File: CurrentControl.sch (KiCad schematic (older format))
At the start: 8 parts, among them P1 CONN_01X01, P3 A, Q401 BUK9575, U201 LMV358

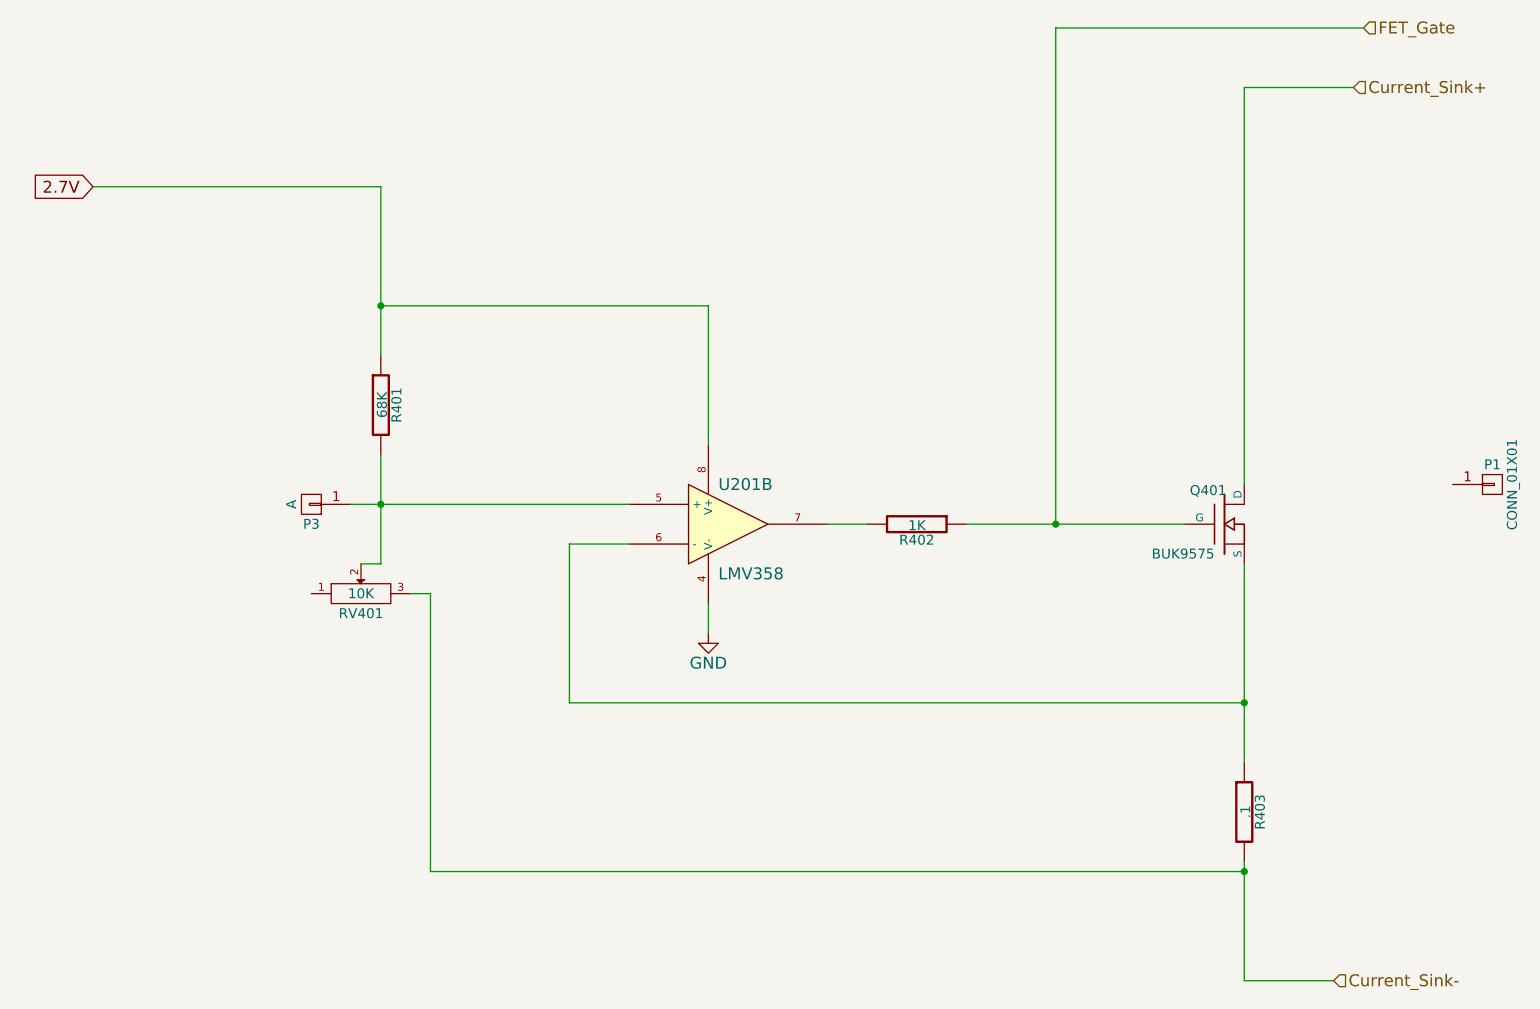
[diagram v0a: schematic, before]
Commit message: test netlist
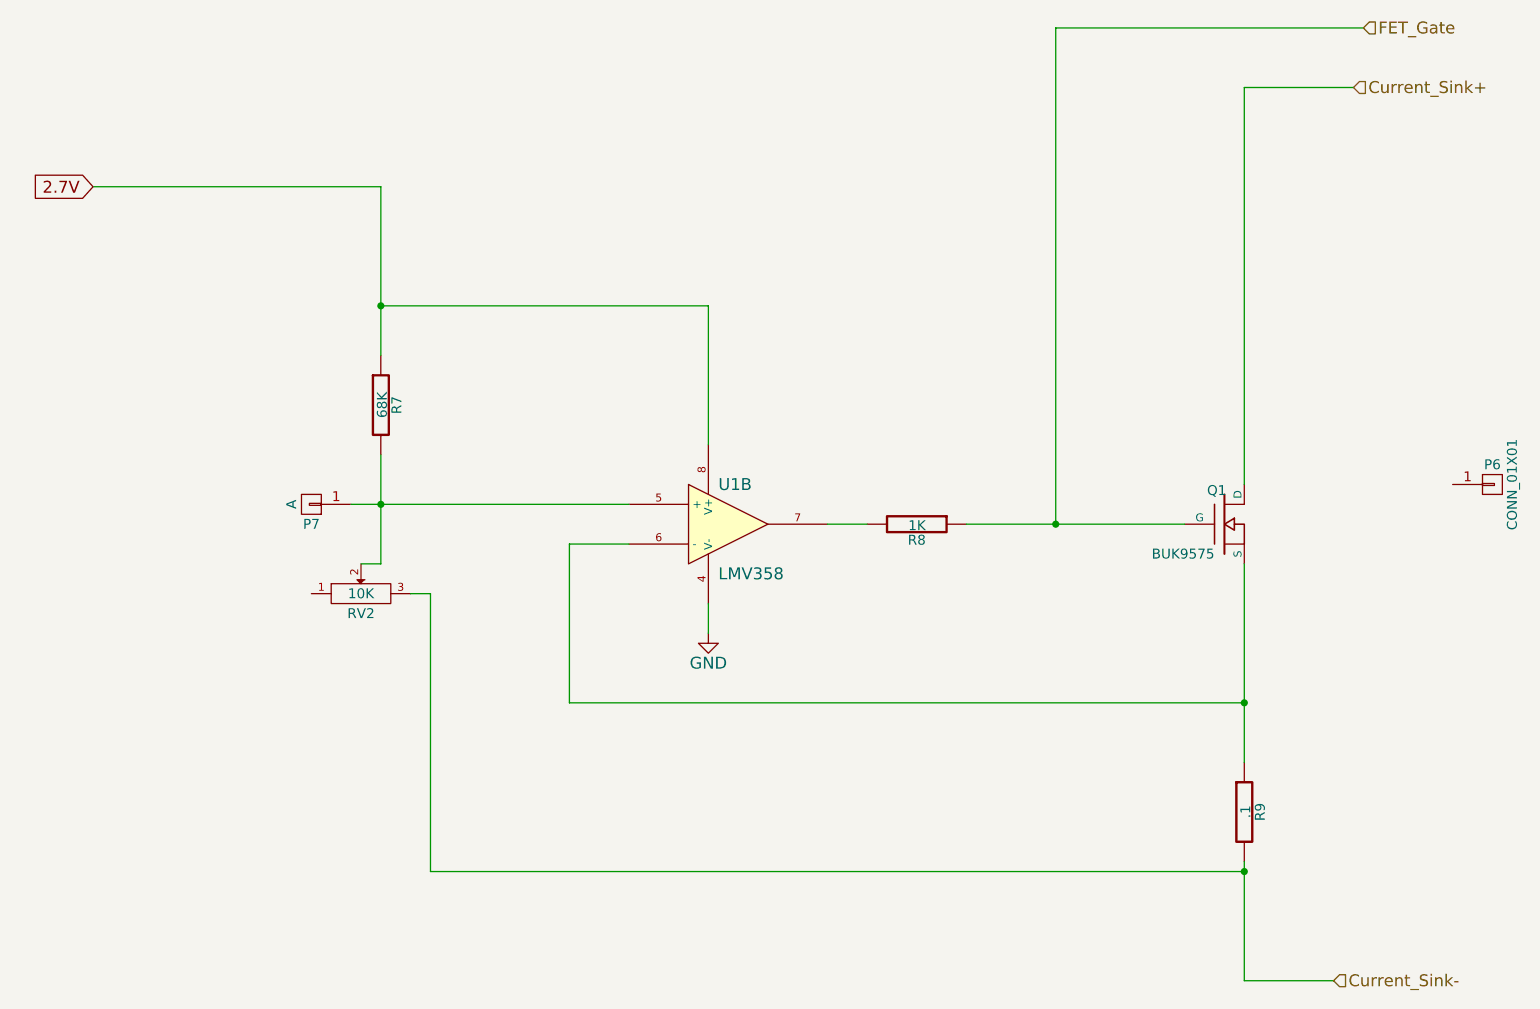
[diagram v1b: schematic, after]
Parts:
- renumbered P1 to P6, P3 to P7, Q401 to Q1, R401 to R7, R402 to R8, R403 to R9, RV401 to RV2, U201 to U1
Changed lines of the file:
@@
 $EndDescr
 $Comp
-L LMV358 U201
+L LMV358 U1
 U 2 1 54DADC5E
 P 5500 3700
-F 0 "U201" H 5450 3900 60  0000 L CNN
+F 0 "U1" H 5450 3900 60  0000 L CNN
 F 1 "LMV358" H 5450 3450 60  0000 L CNN
 F 2 "SMD_Packages:SOIC-8-N" H 5500 3700 60  0001 C CNN
@@
 $EndComp
 $Comp
-L R R403
+L R R9
 U 1 1 54DADC66
 P 8100 5150
-F 0 "R403" V 8180 5150 50  0000 C CNN
+F 0 "R9" V 8180 5150 50  0000 C CNN
 F 1 ".1" V 8107 5151 50  0000 C CNN
 F 2 "Current:1W-Resistor" V 8030 5150 30  0001 C CNN
@@
 $EndComp
 $Comp
-L MOSFET_N Q401
+L MOSFET_N Q1
 U 1 1 54DADC74
 P 8000 3700
-F 0 "Q401" H 8010 3870 50  0000 R CNN
+F 0 "Q1" H 8010 3870 50  0000 R CNN
 F 1 "BUK9575" H 7950 3550 50  0000 R CNN
 F 2 "Current:current-TO-220_FET-GDS_Vertical" H 8000 3700 60  0001 C CNN
@@
 $EndComp
 $Comp
-L GND #PWR07
+L GND #PWR7
 U 1 1 54DADC82
 P 5400 4250
-F 0 "#PWR07" H 5400 4000 60  0001 C CNN
+F 0 "#PWR7" H 5400 4000 60  0001 C CNN
 F 1 "GND" H 5400 4100 60  0000 C CNN
 F 2 "" H 5400 4250 60  0000 C CNN
@@
 Connection ~ 8100 5450
 $Comp
-L POT RV401
+L POT RV2
 U 1 1 54DADC9B
 P 3650 4050
-F 0 "RV401" H 3650 3950 50  0000 C CNN
+F 0 "RV2" H 3650 3950 50  0000 C CNN
 F 1 "10K" H 3650 4050 50  0000 C CNN
 F 2 "Current:P090L-02F25BR10K" H 3650 4050 60  0001 C CNN
@@
 	8650 1500 8100 1500
 $Comp
-L R R402
+L R R8
 U 1 1 54DAE31B
 P 6450 3700
-F 0 "R402" V 6530 3700 50  0000 C CNN
+F 0 "R8" V 6530 3700 50  0000 C CNN
 F 1 "1K" V 6457 3701 50  0000 C CNN
 F 2 "SMD_Packages:SMD-0805" V 6380 3700 30  0001 C CNN
@@
 Current_Sink-
 $Comp
-L CONN_01X01 P1
+L CONN_01X01 P6
 U 1 1 54DFC527
 P 9350 3500
-F 0 "P1" H 9350 3600 50  0000 C CNN
+F 0 "P6" H 9350 3600 50  0000 C CNN
 F 1 "CONN_01X01" V 9450 3500 50  0000 C CNN
 F 2 "Current:FA-T220-38E" H 9350 3500 60  0001 C CNN
@@
 $EndComp
 $Comp
-L R R401
+L R R7
 U 1 1 54DADC7B
 P 3750 3100
-F 0 "R401" V 3830 3100 50  0000 C CNN
+F 0 "R7" V 3830 3100 50  0000 C CNN
 F 1 "68K" V 3757 3101 50  0000 C CNN
 F 2 "SMD_Packages:SMD-0805" V 3680 3100 30  0001 C CNN
@@
 	4000 5450 8100 5450
 $Comp
-L CONN_01X01 P3
+L CONN_01X01 P7
 U 1 1 54F1F408
 P 3400 3600
-F 0 "P3" H 3400 3700 50  0000 C CNN
+F 0 "P7" H 3400 3700 50  0000 C CNN
 F 1 "A" V 3500 3600 50  0000 C CNN
 F 2 "Pin_Headers:Pin_Header_Straight_1x01" H 3400 3600 60  0001 C CNN

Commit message: Revert "Routing done"
This reverts commit 9c8e4a17aa7ae0fb22a7aeeae40aa608407b6119.

Conflicts:
	CurrentSinkOrSwim.sch
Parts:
- Q1: footprint Current:current-TO-220_FET-GDS_Vertical -> Transistors_TO-220:TO-220_FET-GDS_Vertical
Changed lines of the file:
@@
 F 0 "Q1" H 8010 3870 50  0000 R CNN
 F 1 "BUK9575" H 7950 3550 50  0000 R CNN
-F 2 "Current:current-TO-220_FET-GDS_Vertical" H 8000 3700 60  0001 C CNN
+F 2 "Transistors_TO-220:TO-220_FET-GDS_Vertical" H 8000 3700 60  0001 C CNN
 F 3 "" H 8000 3700 60  0000 C CNN
 F 4 "BUK9575-100A,127" H 8000 3700 60  0001 C CNN "MPN"

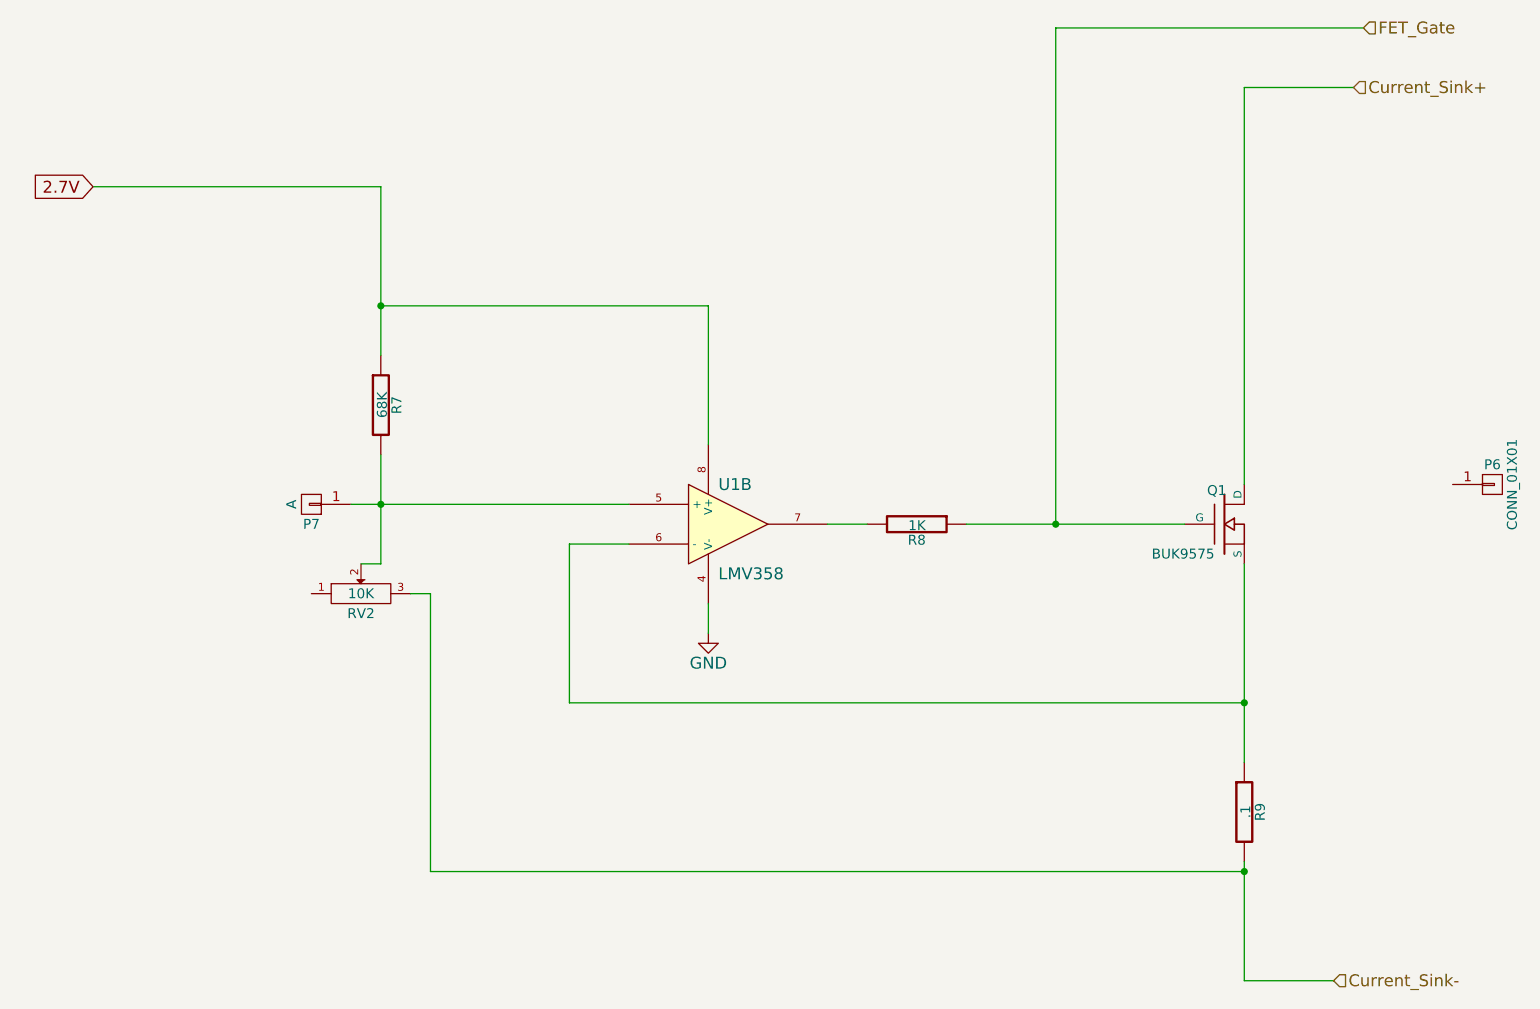
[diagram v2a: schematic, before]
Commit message: Routing done - Final
Just add artwork
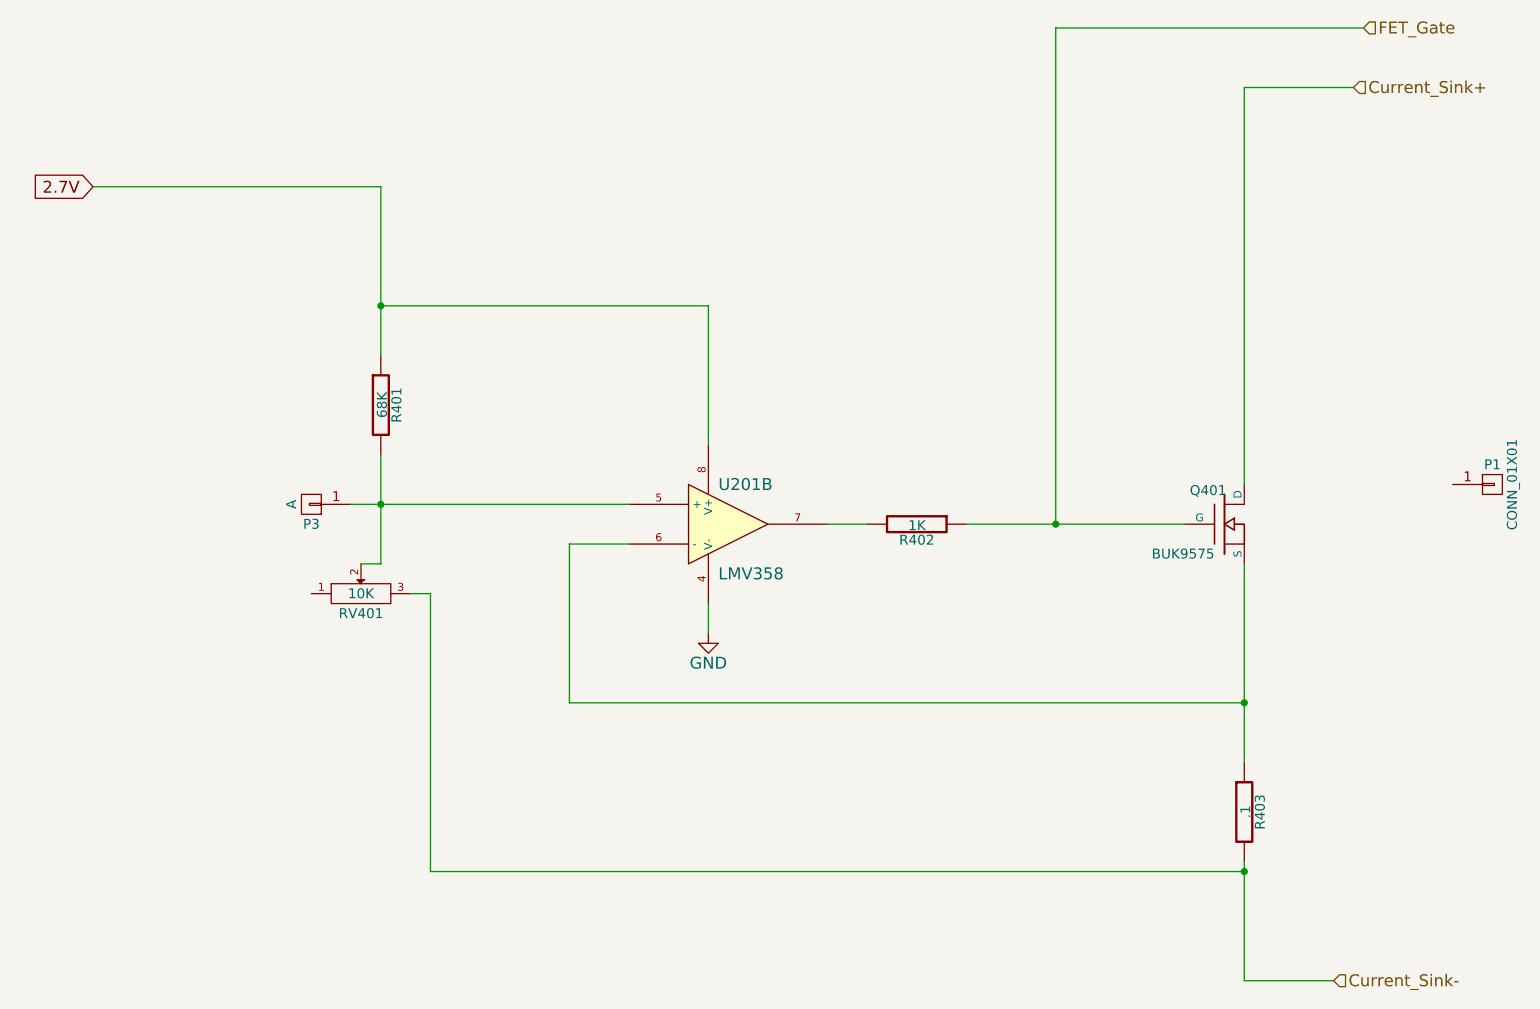
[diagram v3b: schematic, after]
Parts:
- Q401: renamed from Q1; footprint Transistors_TO-220:TO-220_FET-GDS_Vertical -> Current:current-TO-220_FET-GDS_Vertical
- renumbered P6 to P1, P7 to P3, R7 to R401, R8 to R402, R9 to R403, RV2 to RV401, U1 to U201
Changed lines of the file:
@@
 $EndDescr
 $Comp
-L LMV358 U1
+L LMV358 U201
 U 2 1 54DADC5E
 P 5500 3700
-F 0 "U1" H 5450 3900 60  0000 L CNN
+F 0 "U201" H 5450 3900 60  0000 L CNN
 F 1 "LMV358" H 5450 3450 60  0000 L CNN
 F 2 "SMD_Packages:SOIC-8-N" H 5500 3700 60  0001 C CNN
@@
 $EndComp
 $Comp
-L R R9
+L R R403
 U 1 1 54DADC66
 P 8100 5150
-F 0 "R9" V 8180 5150 50  0000 C CNN
+F 0 "R403" V 8180 5150 50  0000 C CNN
 F 1 ".1" V 8107 5151 50  0000 C CNN
 F 2 "Current:1W-Resistor" V 8030 5150 30  0001 C CNN
@@
 $EndComp
 $Comp
-L MOSFET_N Q1
+L MOSFET_N Q401
 U 1 1 54DADC74
 P 8000 3700
-F 0 "Q1" H 8010 3870 50  0000 R CNN
+F 0 "Q401" H 8010 3870 50  0000 R CNN
 F 1 "BUK9575" H 7950 3550 50  0000 R CNN
-F 2 "Transistors_TO-220:TO-220_FET-GDS_Vertical" H 8000 3700 60  0001 C CNN
+F 2 "Current:current-TO-220_FET-GDS_Vertical" H 8000 3700 60  0001 C CNN
 F 3 "" H 8000 3700 60  0000 C CNN
 F 4 "BUK9575-100A,127" H 8000 3700 60  0001 C CNN "MPN"
@@
 $EndComp
 $Comp
-L GND #PWR7
+L GND #PWR07
 U 1 1 54DADC82
 P 5400 4250
-F 0 "#PWR7" H 5400 4000 60  0001 C CNN
+F 0 "#PWR07" H 5400 4000 60  0001 C CNN
 F 1 "GND" H 5400 4100 60  0000 C CNN
 F 2 "" H 5400 4250 60  0000 C CNN
@@
 Connection ~ 8100 5450
 $Comp
-L POT RV2
+L POT RV401
 U 1 1 54DADC9B
 P 3650 4050
-F 0 "RV2" H 3650 3950 50  0000 C CNN
+F 0 "RV401" H 3650 3950 50  0000 C CNN
 F 1 "10K" H 3650 4050 50  0000 C CNN
 F 2 "Current:P090L-02F25BR10K" H 3650 4050 60  0001 C CNN
@@
 	8650 1500 8100 1500
 $Comp
-L R R8
+L R R402
 U 1 1 54DAE31B
 P 6450 3700
-F 0 "R8" V 6530 3700 50  0000 C CNN
+F 0 "R402" V 6530 3700 50  0000 C CNN
 F 1 "1K" V 6457 3701 50  0000 C CNN
 F 2 "SMD_Packages:SMD-0805" V 6380 3700 30  0001 C CNN
@@
 Current_Sink-
 $Comp
-L CONN_01X01 P6
+L CONN_01X01 P1
 U 1 1 54DFC527
 P 9350 3500
-F 0 "P6" H 9350 3600 50  0000 C CNN
+F 0 "P1" H 9350 3600 50  0000 C CNN
 F 1 "CONN_01X01" V 9450 3500 50  0000 C CNN
 F 2 "Current:FA-T220-38E" H 9350 3500 60  0001 C CNN
@@
 $EndComp
 $Comp
-L R R7
+L R R401
 U 1 1 54DADC7B
 P 3750 3100
-F 0 "R7" V 3830 3100 50  0000 C CNN
+F 0 "R401" V 3830 3100 50  0000 C CNN
 F 1 "68K" V 3757 3101 50  0000 C CNN
 F 2 "SMD_Packages:SMD-0805" V 3680 3100 30  0001 C CNN
@@
 	4000 5450 8100 5450
 $Comp
-L CONN_01X01 P7
+L CONN_01X01 P3
 U 1 1 54F1F408
 P 3400 3600
-F 0 "P7" H 3400 3700 50  0000 C CNN
+F 0 "P3" H 3400 3700 50  0000 C CNN
 F 1 "A" V 3500 3600 50  0000 C CNN
 F 2 "Pin_Headers:Pin_Header_Straight_1x01" H 3400 3600 60  0001 C CNN
